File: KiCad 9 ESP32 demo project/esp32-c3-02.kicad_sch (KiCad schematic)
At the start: 30 parts, among them J3 GSD090012SEU, U3 ESP32-C3-WROOM-02-H4, U4 CP2102N-Axx-xQFN20, U5 USBLC6-2SC6, U6 W25Q32JVSSIQ

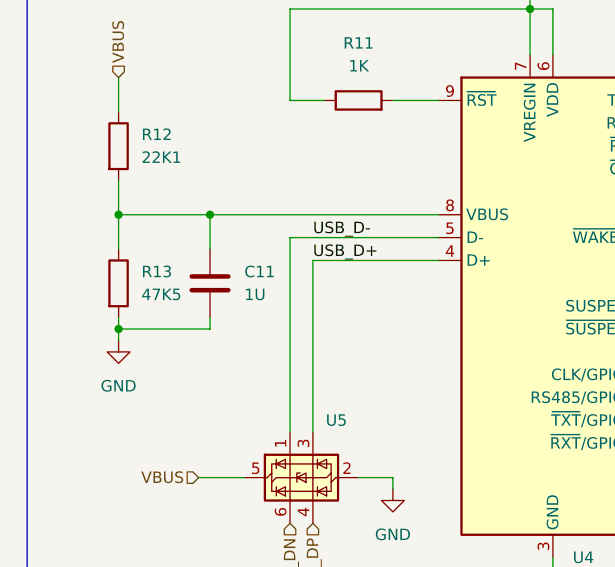
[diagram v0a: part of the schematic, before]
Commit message: power layout done
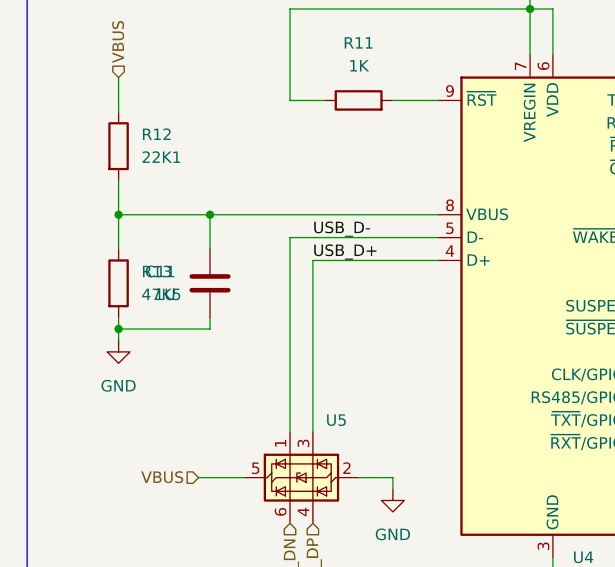
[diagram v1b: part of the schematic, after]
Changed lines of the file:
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@@
 		(lib_id "Device:C")
 		(at 39.37 87.63 0)
+		(mirror y)
 		(unit 1)
 		(exclude_from_sim no)
@@
 		(on_board yes)
 		(dnp no)
-		(fields_autoplaced yes)
 		(property "Reference" "C11"
-			(at 43.18 86.3599 0)
+			(at 35.56 86.3599 0)
 			(effects
 				(font
@@
 		)
 		(property "Value" "1U"
-			(at 43.18 88.8999 0)
+			(at 35.56 88.8999 0)
 			(effects
 				(font
@@
 		)
 		(property "Footprint" "Capacitor_SMD:C_0805_2012Metric"
-			(at 40.3352 91.44 0)
+			(at 38.4048 91.44 0)
 			(effects
 				(font
